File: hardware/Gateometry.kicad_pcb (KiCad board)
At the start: 2 copper layers, 99.6 x 100 mm, 79 parts, among them J1 GATE1, J10 CLOCK IN, J11 POWER, J2 GATE2, J3 GATE3, J4 GATE4, J5 GATE5, J6 GATE6, J7 GATE7, J8 GATE8, J9 CLOCK OUT, SW1 RUN/STOP, SW2 MUTE1, SW3 MUTE2, SW4 MUTE3, SW5 MUTE4, SW6 MUTE5, SW7 MUTE6, SW8 MUTE7, SW9 MUTE8, U1 74HC595, U2 74HCT541, U3 0.96 Inch OLED I2C Display Mo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, U4 74HCT541, U5 74HCT14, U6 74HC165

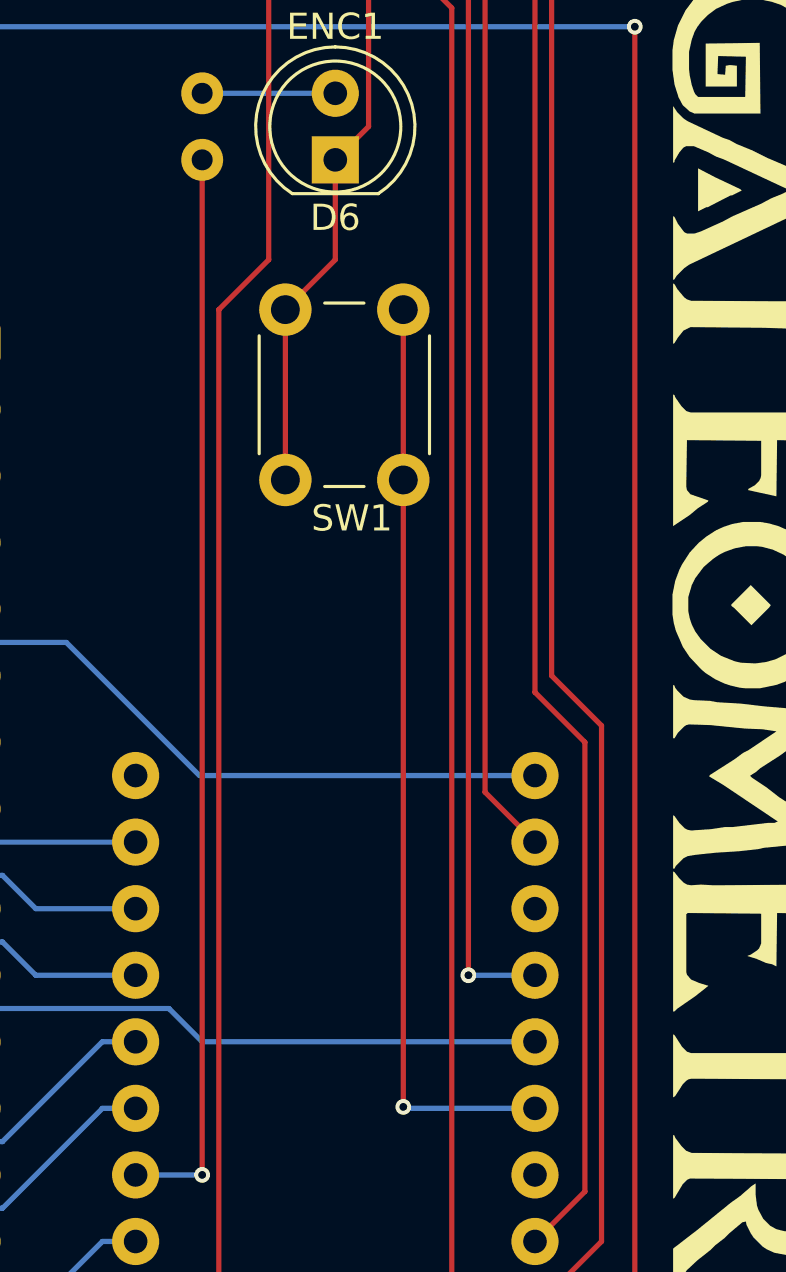
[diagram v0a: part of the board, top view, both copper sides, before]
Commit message: panel work
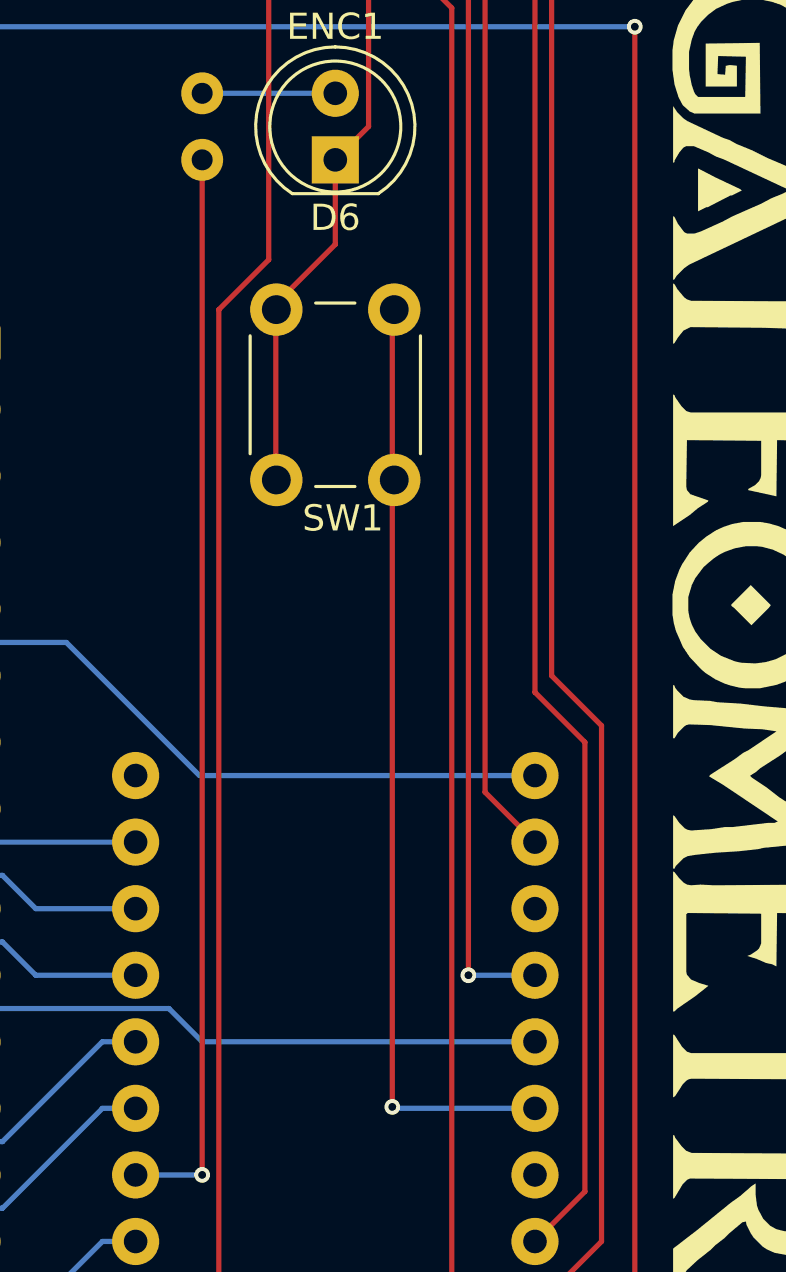
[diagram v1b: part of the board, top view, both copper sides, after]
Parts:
- moved SW1 0.34 mm to (170.4, 84.8)
